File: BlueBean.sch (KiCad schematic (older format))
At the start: 1 part, among them U7 BLUE-BEAN

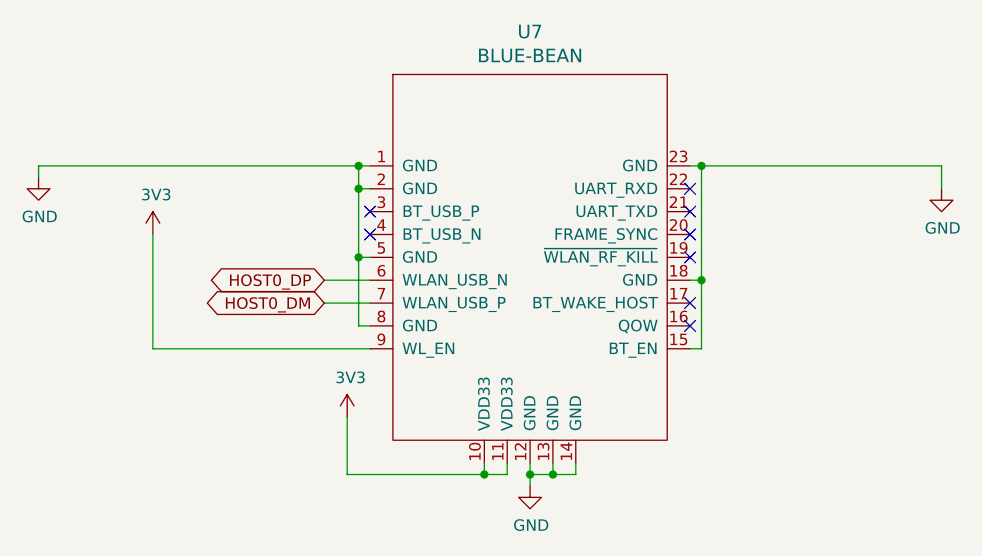
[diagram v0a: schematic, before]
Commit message: started layout of the PCB, allso moved onto craken rum, from captin morgan. please for the love of god check the footprints are right. @MAX
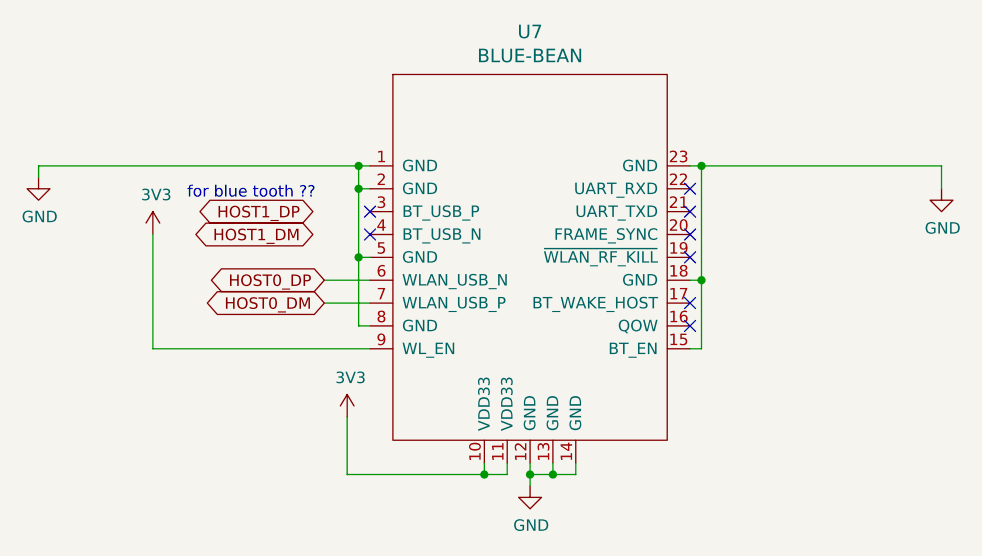
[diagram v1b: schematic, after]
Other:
- note added: "for blue tooth ??"
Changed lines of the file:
@@
 	1    0    0    -1
 $EndComp
+Text GLabel 3400 3100 0    50   BiDi ~ 0
+HOST1_DM
+Text GLabel 3400 3000 0    50   BiDi ~ 0
+HOST1_DP
+Text Notes 2850 2950 0    50   ~ 0
+for blue tooth ??
 $EndSCHEMATC
